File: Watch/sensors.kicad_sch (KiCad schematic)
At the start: 15 parts, among them U2 MAX30102EFD+T, U4 TMP117AIDRVT, U8 LSM6DSV80XTR

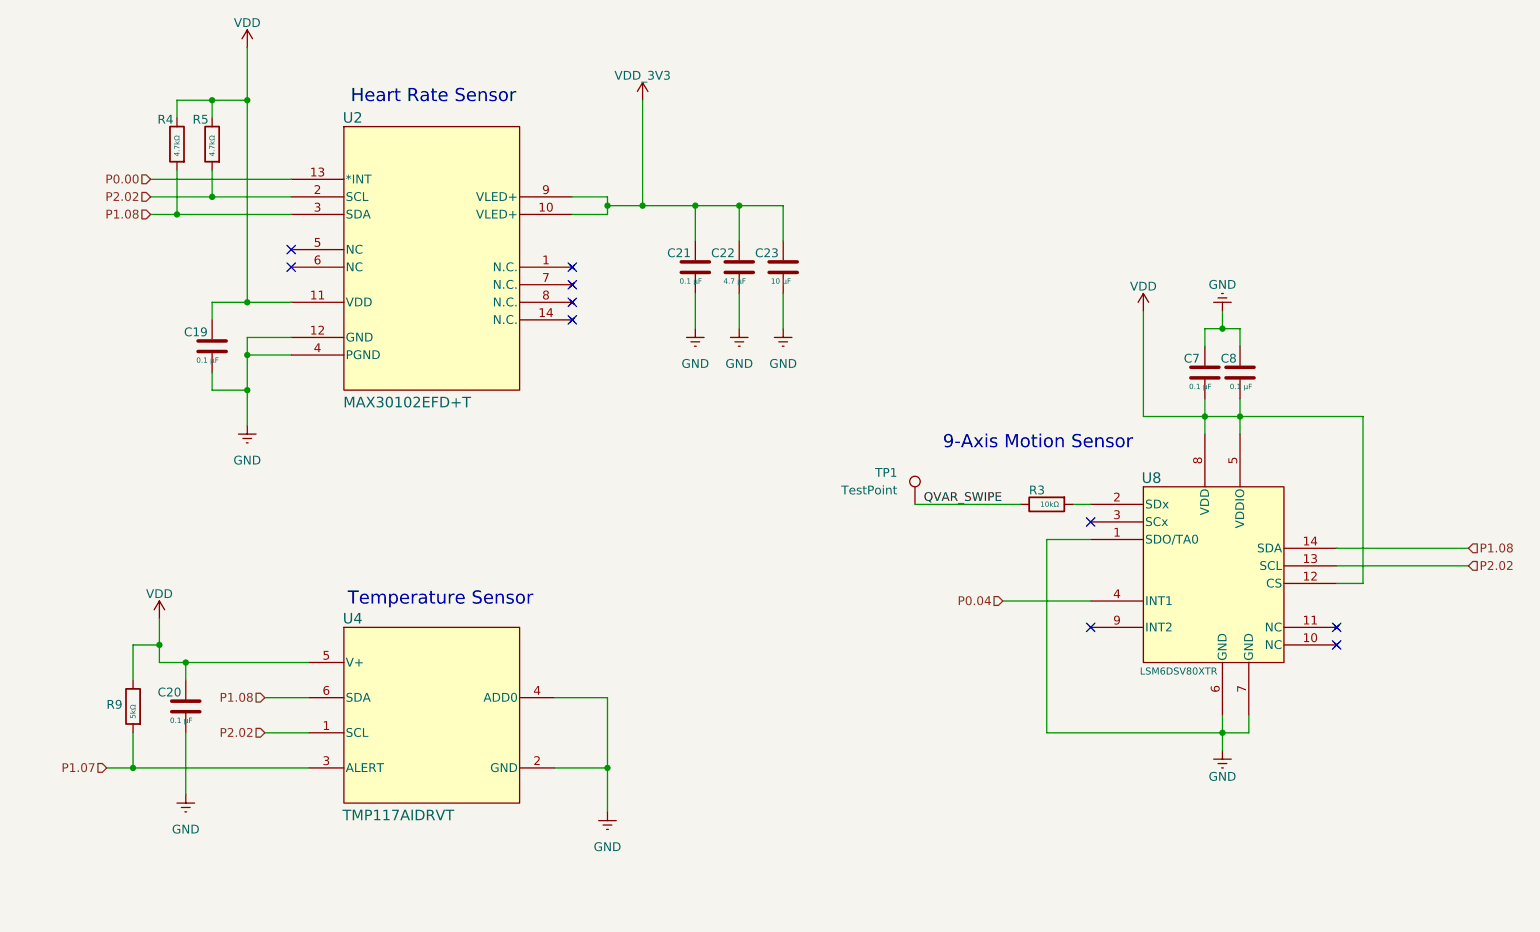
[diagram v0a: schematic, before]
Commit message: Screenshots
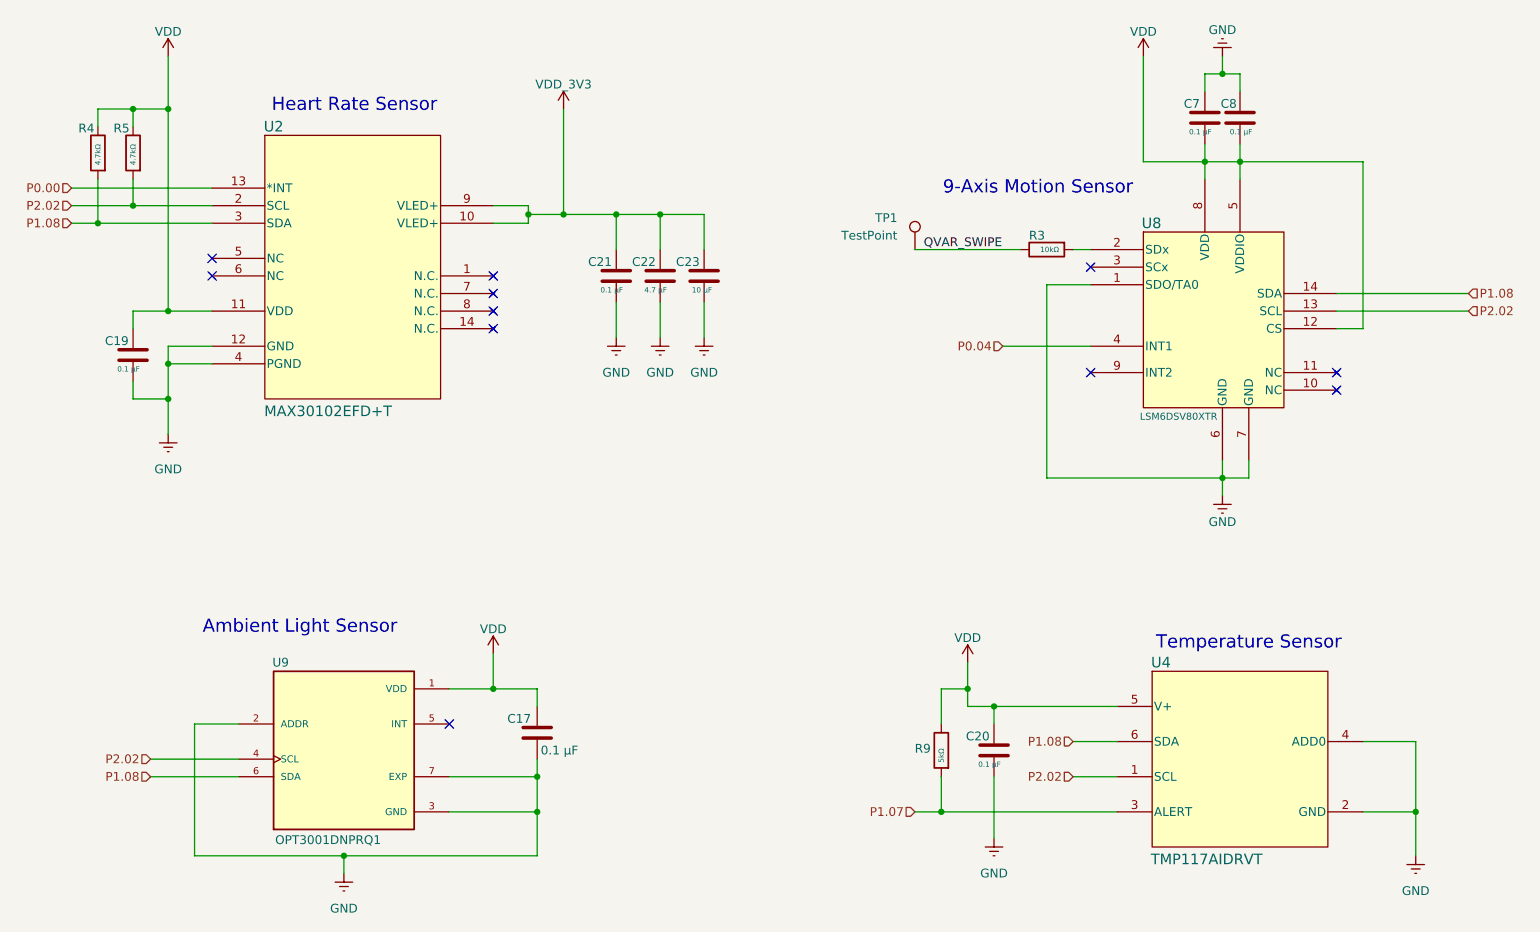
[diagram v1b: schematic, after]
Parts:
- added C17: 0.1 μF, Capacitor_SMD:C_0402_1005Metric, symbol Device:C
- added U9: OPT3001DNPRQ1, 1_I_Syst.inc:SON65P200X200X65-7N, symbol I_Syst_inc:OPT3001DNPRQ1
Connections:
- net GND: now also C17.2, U9.2 (ADDR), U9.3 (GND), U9.7 (EXP)
- net P1.08: now also U9.6 (SDA)
- net P2.02: now also U9.4 (SCL)
- net VDD: now also C17.1, U9.1 (VDD)
- no-connect marks 10 -> 11
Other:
- note added: "Ambient Light Sensor"
- moved on the sheet: C19, C20, C21, C22, C23, C7, C8, R3, R4, R5, R9, TP1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
